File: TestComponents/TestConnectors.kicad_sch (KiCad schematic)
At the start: 8 parts, among them J2-1 Conn_01x04_Male, J2-2 Conn_01x04_Male

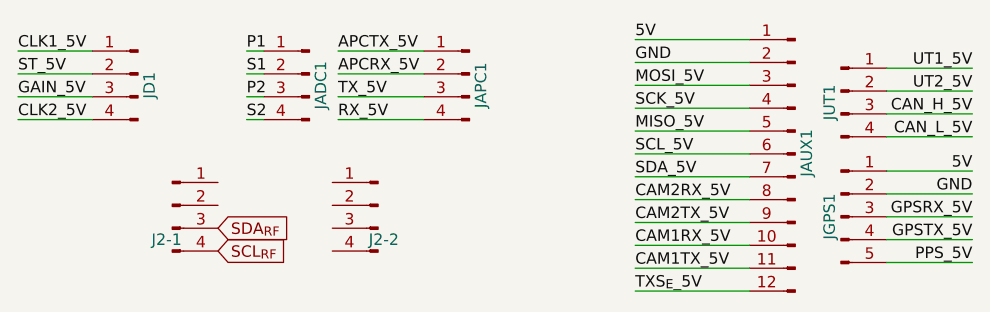
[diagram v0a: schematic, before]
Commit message: SpectDrone Development
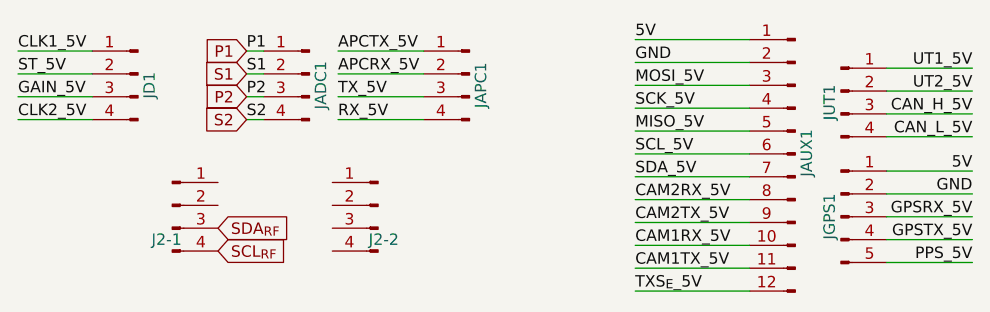
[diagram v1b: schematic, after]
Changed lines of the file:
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@@
     (effects (font (size 1.27 1.27)) (justify right bottom))
+  )
+  (global_label "S1" (shape input) (at 125.095 90.805 180) (fields_autoplaced)
+    (effects (font (size 1.27 1.27)) (justify right))
+    (property "Intersheet References" "${INTERSHEET_REFS}" (id 0) (at 120.2629 90.7256 0)
+      (effects (font (size 1.27 1.27)) (justify right) hide)
+    )
+  )
+  (global_label "P1" (shape input) (at 125.095 88.265 180) (fields_autoplaced)
+    (effects (font (size 1.27 1.27)) (justify right))
+    (property "Intersheet References" "${INTERSHEET_REFS}" (id 0) (at 120.2024 88.1856 0)
+      (effects (font (size 1.27 1.27)) (justify right) hide)
+    )
+  )
+  (global_label "P2" (shape input) (at 125.095 93.345 180) (fields_autoplaced)
+    (effects (font (size 1.27 1.27)) (justify right))
+    (property "Intersheet References" "${INTERSHEET_REFS}" (id 0) (at 120.2024 93.2656 0)
+      (effects (font (size 1.27 1.27)) (justify right) hide)
+    )
   )
   (global_label "SDA_{RF}" (shape input) (at 121.92 107.95 0) (fields_autoplaced)
@@
     )
   )
+  (global_label "S2" (shape input) (at 125.095 95.885 180) (fields_autoplaced)
+    (effects (font (size 1.27 1.27)) (justify right))
+    (property "Intersheet References" "${INTERSHEET_REFS}" (id 0) (at 120.2629 95.8056 0)
+      (effects (font (size 1.27 1.27)) (justify right) hide)
+    )
+  )

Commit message: SpectDrone Development
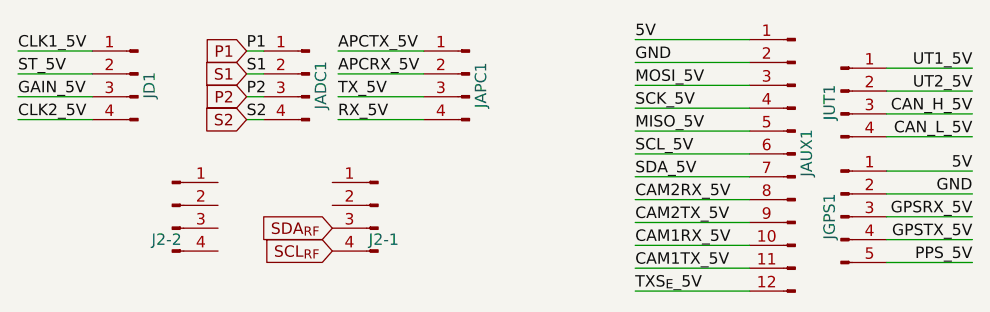
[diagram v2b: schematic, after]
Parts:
- renumbered J2-2 to J2-1, J2-1 to J2-2
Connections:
- net SCL_{RF}: now also J2-1.4 (Pin_4); no longer J2-2.4 (Pin_4)
- net SDA_{RF}: now also J2-1.3 (Pin_3); no longer J2-2.3 (Pin_3)
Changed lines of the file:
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@@
     )
   )
-  (global_label "SDA_{RF}" (shape input) (at 121.92 107.95 0) (fields_autoplaced)
-    (effects (font (size 1.27 1.27)) (justify left))
-    (property "Intersheet References" "${INTERSHEET_REFS}" (id 0) (at 129.7881 108.0294 0)
-      (effects (font (size 1.27 1.27)) (justify left) hide)
+  (global_label "SDA_{RF}" (shape input) (at 134.62 107.95 180) (fields_autoplaced)
+    (effects (font (size 1.27 1.27)) (justify right))
+    (property "Intersheet References" "${INTERSHEET_REFS}" (id 0) (at 126.7519 108.0294 0)
+      (effects (font (size 1.27 1.27)) (justify right) hide)
     )
   )
-  (global_label "SCL_{RF}" (shape input) (at 121.92 110.49 0) (fields_autoplaced)
-    (effects (font (size 1.27 1.27)) (justify left))
-    (property "Intersheet References" "${INTERSHEET_REFS}" (id 0) (at 129.7276 110.5694 0)
-      (effects (font (size 1.27 1.27)) (justify left) hide)
+  (global_label "SCL_{RF}" (shape input) (at 134.62 110.49 180) (fields_autoplaced)
+    (effects (font (size 1.27 1.27)) (justify right))
+    (property "Intersheet References" "${INTERSHEET_REFS}" (id 0) (at 126.8124 110.5694 0)
+      (effects (font (size 1.27 1.27)) (justify right) hide)
     )
   )
@@
   (symbol (lib_id "Connector:Conn_01x04_Male") (at 116.84 105.41 0) (unit 1)
     (in_bom yes) (on_board yes)
-    (property "Reference" "J2-1" (id 0) (at 116.205 109.22 0))
+    (property "Reference" "J2-2" (id 0) (at 116.205 109.22 0))
     (property "Value" "Conn_01x04_Male" (id 1) (at 127 106.68 0)
       (effects (font (size 1.27 1.27)) hide)
@@
   (symbol (lib_id "Connector:Conn_01x04_Male") (at 139.7 105.41 0) (mirror y) (unit 1)
     (in_bom yes) (on_board yes)
-    (property "Reference" "J2-2" (id 0) (at 140.335 109.22 0))
+    (property "Reference" "J2-1" (id 0) (at 140.335 109.22 0))
     (property "Value" "Conn_01x04_Male" (id 1) (at 129.54 106.68 0)
       (effects (font (size 1.27 1.27)) hide)
